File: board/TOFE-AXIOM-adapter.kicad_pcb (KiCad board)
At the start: 2 copper layers, 68.9 x 28.3 mm, 8 parts, among them CN1 C, U1 24AA01/24LC01B

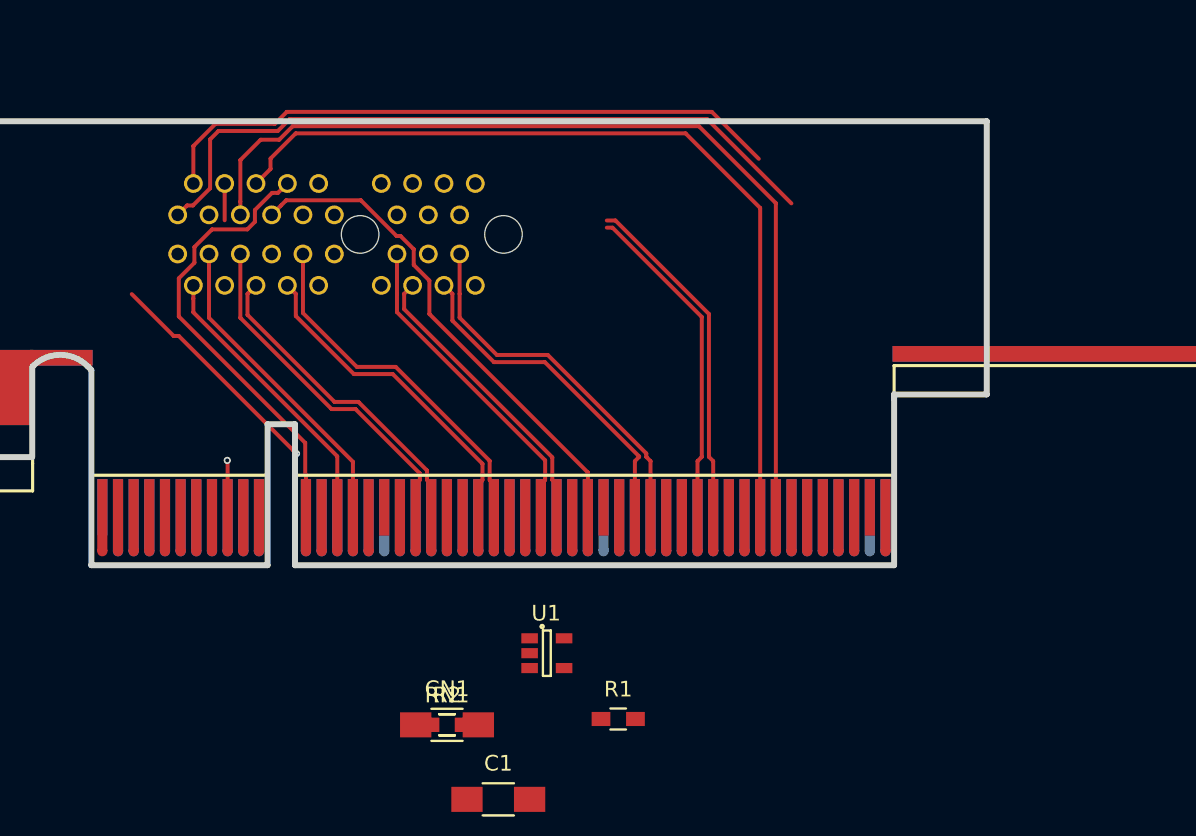
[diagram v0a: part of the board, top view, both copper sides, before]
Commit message: Routing.
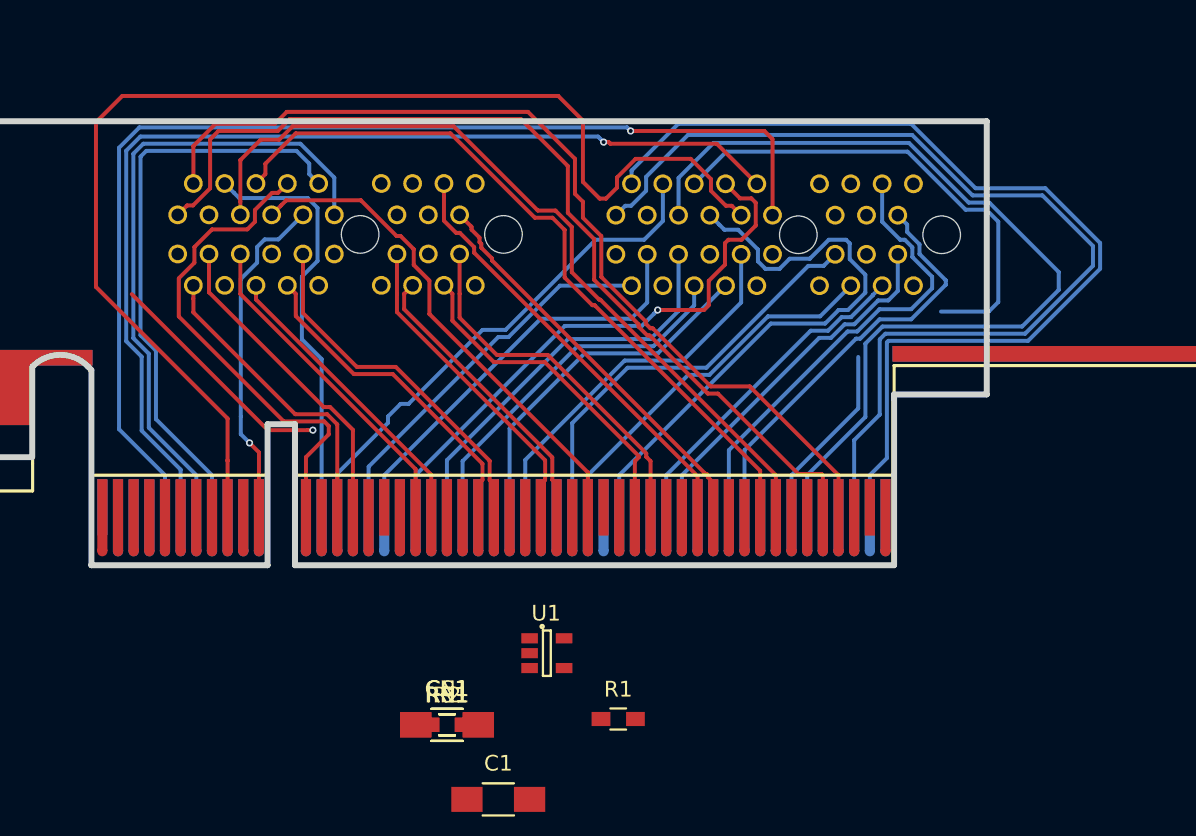
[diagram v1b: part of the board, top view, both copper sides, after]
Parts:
- added CS1: C, Capacitors_SMD:C_1206_HandSoldering, F.Cu at (196.7, 198.3)
- added RS1: R, Resistors_SMD:R_0603_HandSoldering, F.Cu at (196.7, 198.3)
- added SOUTH1: AXIOM-PCIE, w_conn_pc:pci-x_conn-x1, B.Cu at (217.0, 167.1)
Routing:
- net /S_IO5: track 3.51 -> 78.9 mm, vias 1 -> 0
- net /S_IO7: track 0.00 -> 72.1 mm, vias 0 -> 1
- net /S_IO6: track 0.00 -> 66.6 mm, vias 0 -> 1
- net /S_SDA: track 0.00 -> 64.8 mm
- net /S_SCL: track 0.00 -> 63.8 mm
- net /S_IO1: track 0.00 -> 58.4 mm
- net /S_IO2: track 0.00 -> 43.0 mm
- net /N_IO7: track 0.00 -> 41.1 mm
- net /S_IO3: track 0.00 -> 38.3 mm
- net /N_IO6: track 0.00 -> 37.6 mm
- net /S_IO4: track 0.00 -> 36.5 mm, vias 0 -> 1
- net /S_IO0: track 0.00 -> 32.7 mm
- net /S_LVDS_5_P: track 0.00 -> 29.6 mm
- net /S_LVDS_3_P: track 0.00 -> 27.1 mm
- net /S_LVDS_5_N: track 0.00 -> 27.1 mm
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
